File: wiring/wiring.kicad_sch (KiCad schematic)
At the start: 2 parts

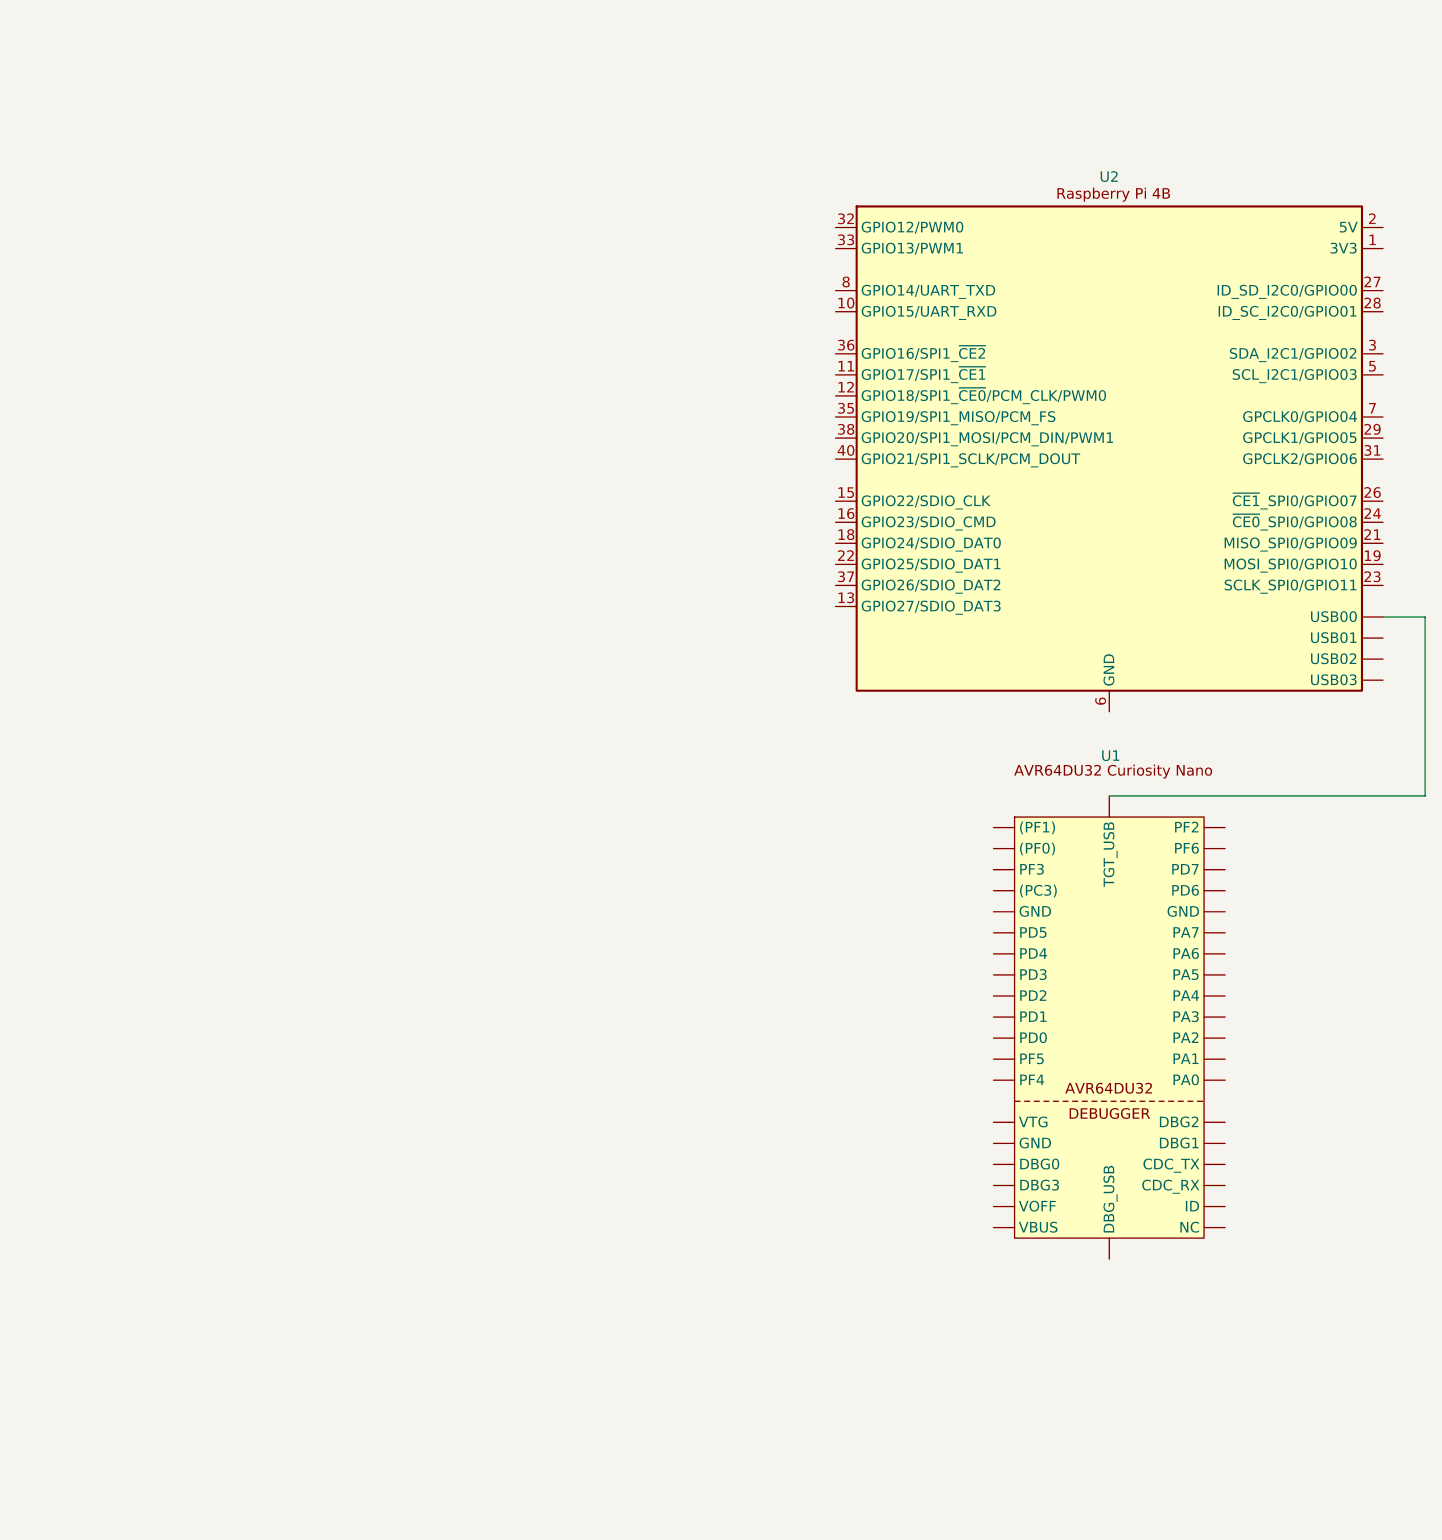
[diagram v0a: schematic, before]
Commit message: completed kicad diagram
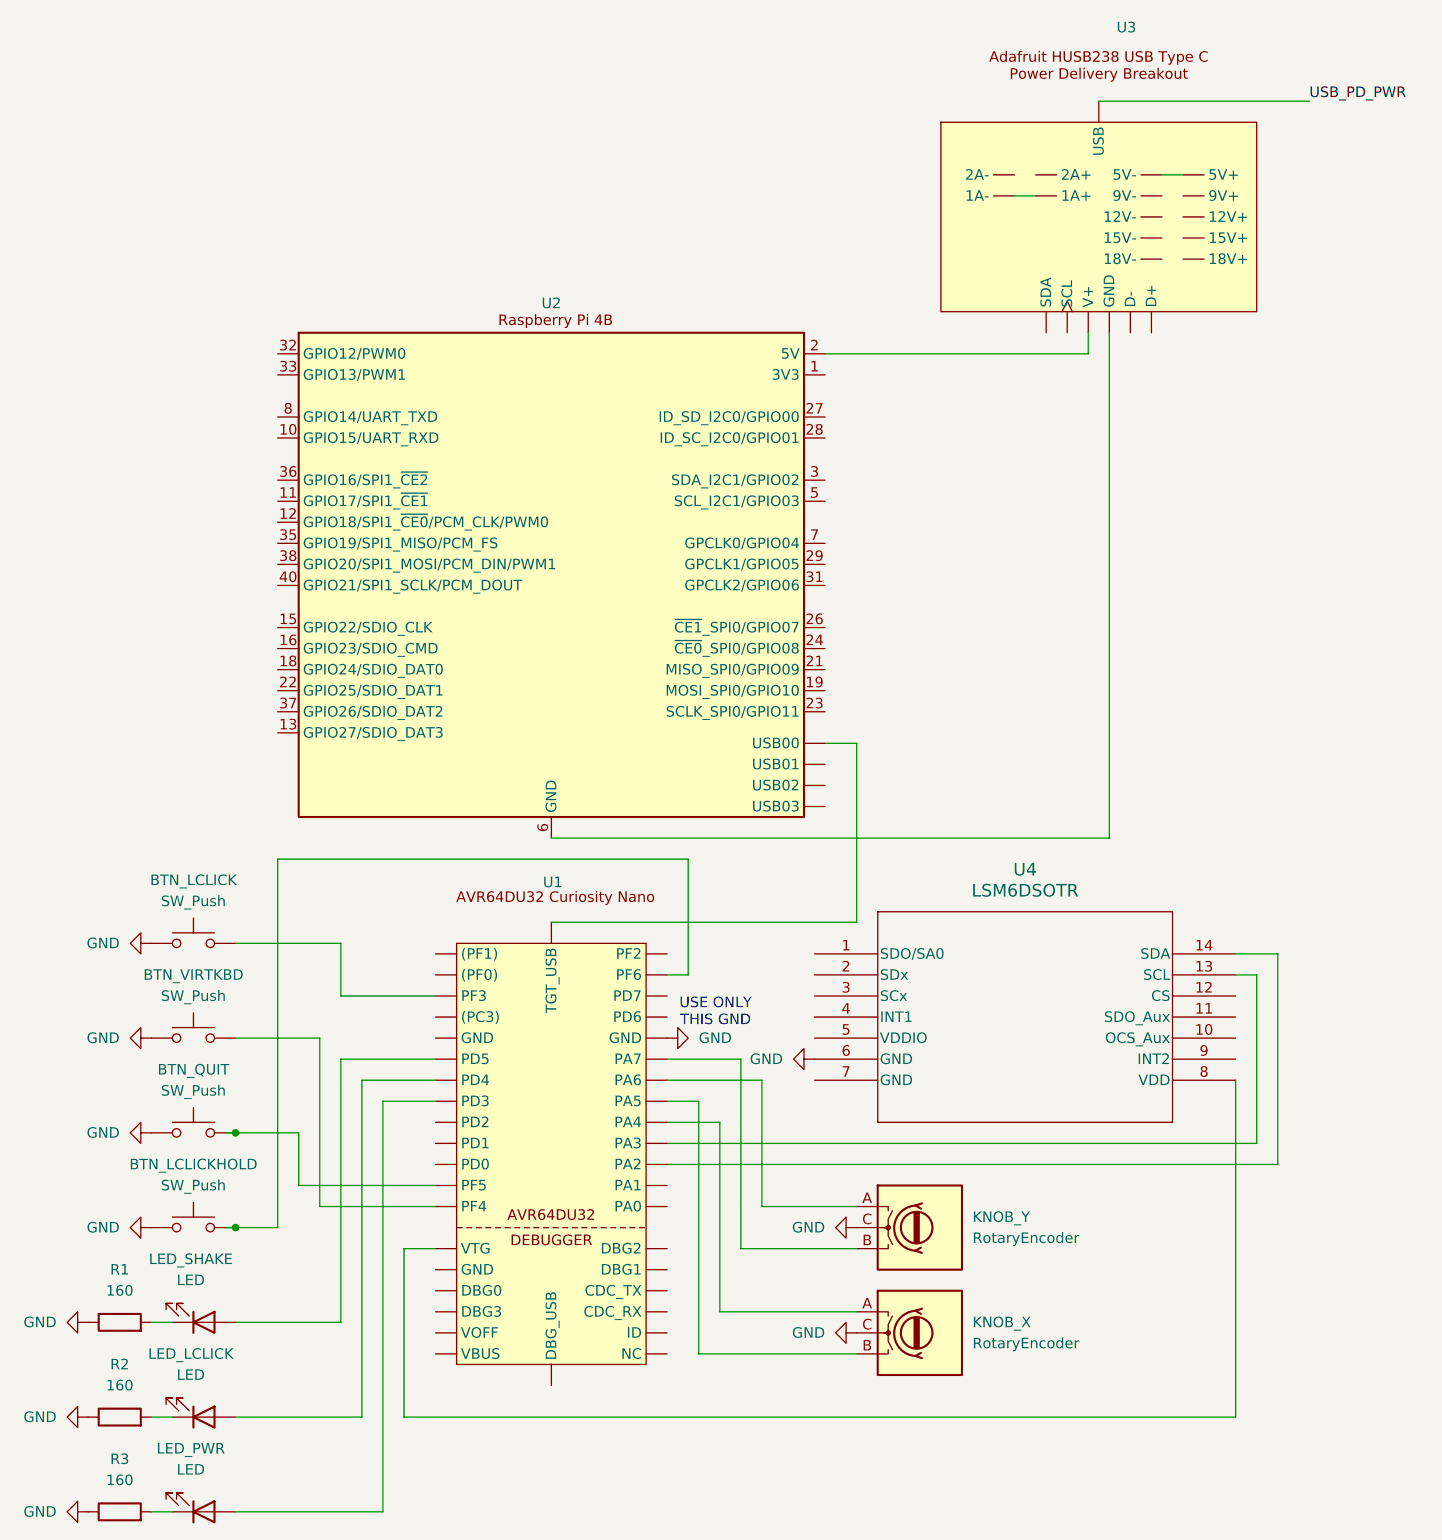
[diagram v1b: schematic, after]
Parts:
- added BTN_LCLICK, BTN_LCLICKHOLD, BTN_QUIT, BTN_VIRTKBD: SW_Push, symbol Switch:SW_Push
- added KNOB_X, KNOB_Y: RotaryEncoder, symbol Device:RotaryEncoder
- added LED_LCLICK, LED_PWR, LED_SHAKE: LED, symbol Device:LED
- added R1, R2, R3: 160, symbol Device:R
- added U3: (no value), symbol CustomSymbols:Adafruit_HUSB238_USB_Type_C_Power_Delivery_Breakout
- added U4: LSM6DSOTR, LGA-14L_2P5X3X0P86_STM, symbol LSM6DSO:LSM6DSOTR
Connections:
- net GND: now reaches U1. (NC)
- net GND: now also BTN_LCLICK.1, BTN_LCLICKHOLD.1, BTN_QUIT.1, BTN_VIRTKBD.1, KNOB_X.C, KNOB_Y.C, R1.1, R2.1, R3.1, U4.6 (GND)
- net at U2. (USB03): no longer U1. (NC)
- net at U2.14 (GND), U2.20 (GND), U2.25 (GND)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: now also U3. (18V+)
- net at U2.2 (5V), U2.4 (5V): now also U3. (18V+)
- new net: LED_SHAKE.1 (K), R1.2
- new net: LED_SHAKE.2 (A), U1. (NC)
- new net: U1. (NC), U4.13 (SCL)
- new net: U1. (NC), U4.14 (SDA)
- new net: U1. (NC), U4.8 (VDD)
- new net: LED_PWR.1 (K), R3.2
- new net: LED_LCLICK.1 (K), R2.2
- new net: LED_LCLICK.2 (A), U1. (NC)
- new net: U1. (NC), U2. (USB03)
- new net: BTN_VIRTKBD.2, U1. (NC)
- new net: BTN_LCLICK.2, U1. (NC)
- new net: LED_PWR.2 (A), U1. (NC)
- new net: KNOB_X.A, U1. (NC)
- new net: KNOB_X.B, U1. (NC)
- new net: BTN_LCLICKHOLD.2, U1. (NC)
- new net: KNOB_Y.A, U1. (NC)
- new net: KNOB_Y.B, U1. (NC)
- new net: BTN_QUIT.2, U1. (NC)
- new net USB_PD_PWR: U3. (18V+)
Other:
- note added: "USE ONLY THIS GND"
- moved on the sheet: U1, U2
